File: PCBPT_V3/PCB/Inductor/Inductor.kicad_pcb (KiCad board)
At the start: 2 copper layers, 15 x 23 mm, 0 parts

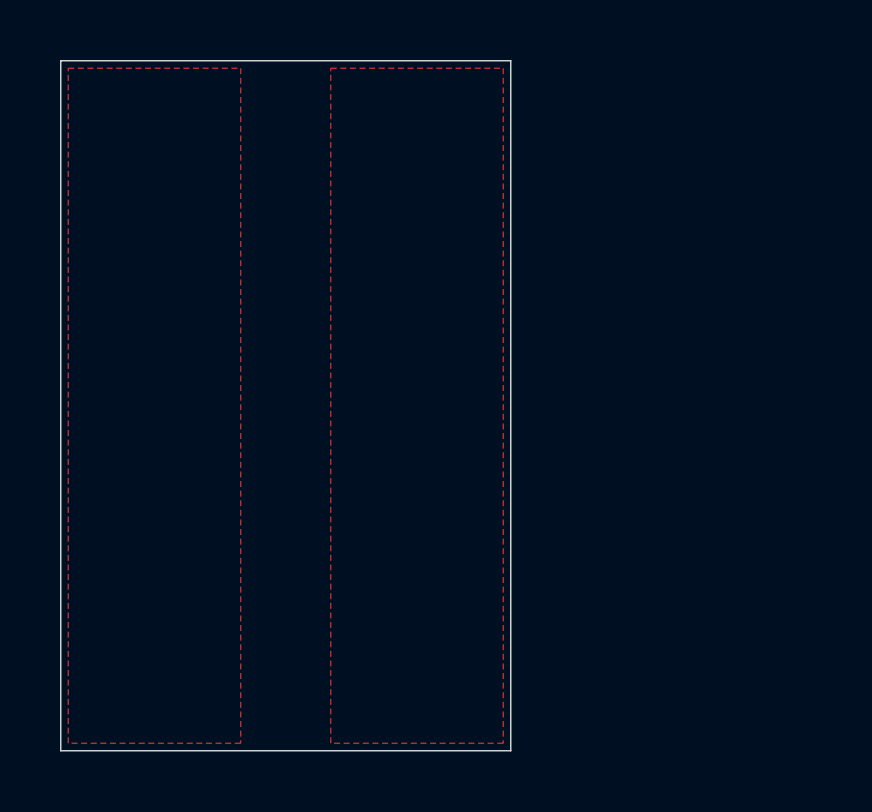
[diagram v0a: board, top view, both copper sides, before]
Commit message: udated by FZ
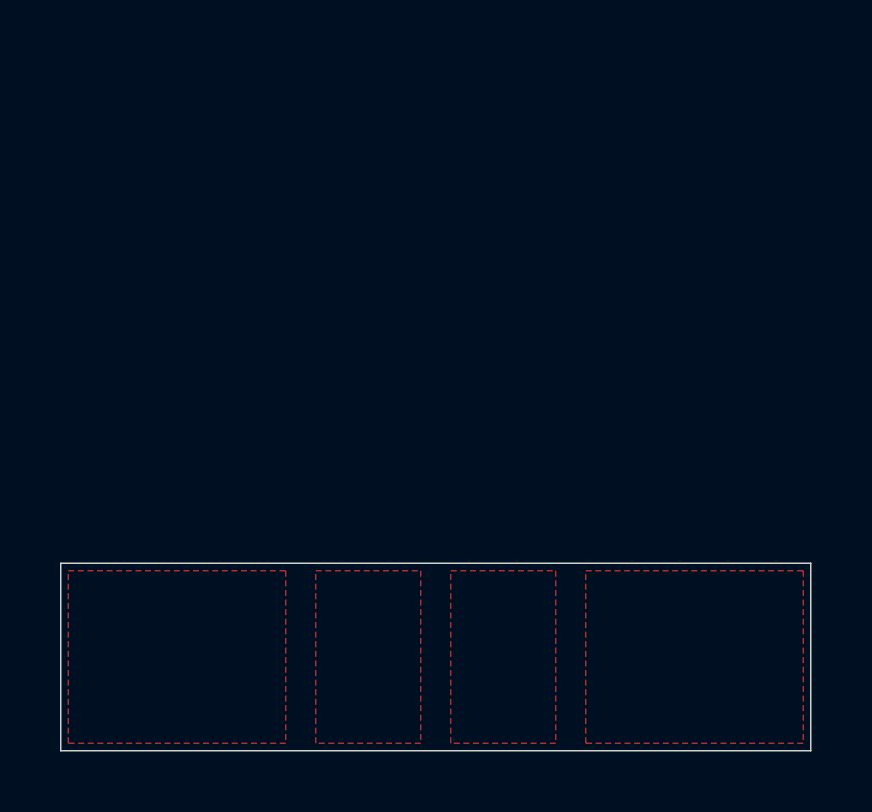
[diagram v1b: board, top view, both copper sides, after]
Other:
- board size 15 x 23 mm -> 25 x 6.2 mm
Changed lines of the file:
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@@
   )
   (net 0 "")
-  (gr_rect (start 120 88.5) (end 135 111.5)
+  (gr_rect (start 120 105.25) (end 145 111.5)
     (stroke (width 0.05) (type default)) (fill none) (layer "Edge.Cuts"))
   (zone (net 0) (net_name "") (layer "F.Cu") (hatch edge 0.5)
@@
     (polygon
       (pts
-        (xy 129 88.75)
-        (xy 134.75 88.75)
-        (xy 134.75 111.25)
-        (xy 129 111.25)
+        (xy 120.25 105.5)
+        (xy 127.5 105.5)
+        (xy 127.5 111.25)
+        (xy 120.25 111.25)
       )
     )
@@
     (polygon
       (pts
-        (xy 120.25 88.75)
-        (xy 126 88.75)
-        (xy 126 111.25)
-        (xy 120.25 111.25)
+        (xy 133 105.5)
+        (xy 136.5 105.5)
+        (xy 136.5 111.25)
+        (xy 133 111.25)
       )
     )
+  )
+  (zone (net 0) (net_name "") (layer "F.Cu") (hatch edge 0.5)
+    (connect_pads (clearance 0.5))
+    (min_thickness 0.25) (filled_areas_thickness no)
+    (fill yes (thermal_gap 0.5) (thermal_bridge_width 0.5) (island_removal_mode 1) (island_area_min 10))
+    (polygon
+      (pts
+        (xy 137.5 105.5)
+        (xy 144.75 105.5)
+        (xy 144.75 111.25)
+        (xy 137.5 111.25)
+      )
+    )
+  )
+  (zone (net 0) (net_name "") (layer "F.Cu") (hatch edge 0.5)
+    (connect_pads (clearance 0.5))
+    (min_thickness 0.25) (filled_areas_thickness no)
+    (fill yes (thermal_gap 0.5) (thermal_bridge_width 0.5) (island_removal_mode 1) (island_area_min 10))
+    (polygon
+      (pts
+        (xy 128.5 105.5)
+        (xy 132 105.5)
+        (xy 132 111.25)
+        (xy 128.5 111.25)
+      )
+    )
